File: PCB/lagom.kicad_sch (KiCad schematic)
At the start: 165 parts, among them J1 Conn_01x04, J2 Conn_01x03, SW1 KEYSW, SW10 KEYSW, SW11 KEYSW, SW12 KEYSW, SW13 KEYSW, SW14 KEYSW, SW15 KEYSW, SW16 KEYSW, SW17 KEYSW, SW18 KEYSW, SW19 KEYSW, SW2 KEYSW, SW20 KEYSW, SW21 KEYSW, SW22 KEYSW, SW23 KEYSW, SW24 KEYSW, SW25 KEYSW, SW26 KEYSW, SW27 KEYSW, SW28 KEYSW, SW29 KEYSW, SW3 KEYSW, SW30 KEYSW, SW31 KEYSW, SW32 KEYSW, SW33 KEYSW, SW34 KEYSW, SW35 KEYSW, SW36 KEYSW, SW37 KEYSW, SW38 KEYSW, SW39 KEYSW, SW4 KEYSW, SW40 KEYSW, SW41 KEYSW, SW42 KEYSW, SW43 KEYSW, SW44 KEYSW, SW45 KEYSW, SW46 KEYSW, SW47 KEYSW, SW48 KEYSW, SW49 KEYSW, SW5 KEYSW, SW50 KEYSW, SW51 KEYSW, SW52 KEYSW, SW53 KEYSW, SW54 KEYSW, SW55 KEYSW, SW56 KEYSW, SW57 KEYSW, SW58 KEYSW, SW59 KEYSW, SW6 KEYSW, SW60 KEYSW, SW61 KEYSW, SW62 KEYSW, SW63 KEYSW, SW64 KEYSW, SW65 KEYSW, SW66 KEYSW, SW67 KEYSW, SW68 KEYSW, SW69 KEYSW, SW7 KEYSW, SW70 KEYSW, SW71 KEYSW, SW72 KEYSW, SW73 KEYSW, SW74 KEYSW, SW75 KEYSW, SW76 KEYSW, SW77 KEYSW, SW78 KEYSW, SW79 KEYSW, SW8 KEYSW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

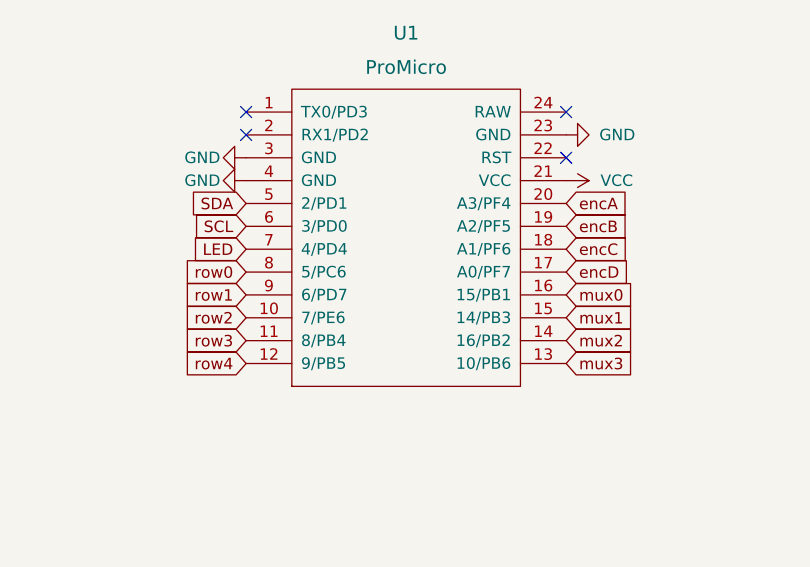
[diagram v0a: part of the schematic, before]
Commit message: PCB mostly done
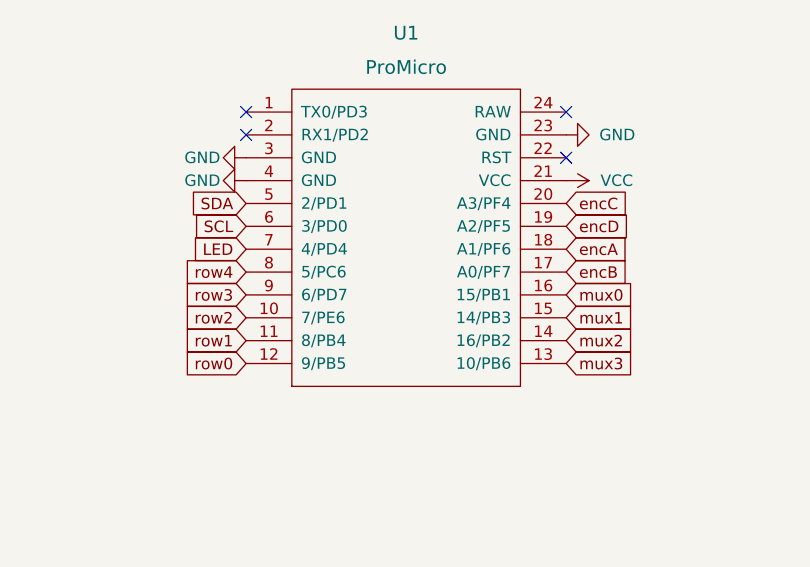
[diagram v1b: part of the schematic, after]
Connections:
- net encA: now also U1.18 (A1/PF6); no longer U1.20 (A3/PF4)
- net encB: now also U1.17 (A0/PF7); no longer U1.19 (A2/PF5)
- net encC: now also U1.20 (A3/PF4); no longer U1.18 (A1/PF6)
- net encD: now also U1.19 (A2/PF5); no longer U1.17 (A0/PF7)
- net row0: now also U1.12 (9/PB5); no longer U1.8 (5/PC6)
- net row1: now also U1.11 (8/PB4); no longer U1.9 (6/PD7)
- net row3: now also U1.9 (6/PD7); no longer U1.11 (8/PB4)
- net row4: now also U1.8 (5/PC6); no longer U1.12 (9/PB5)

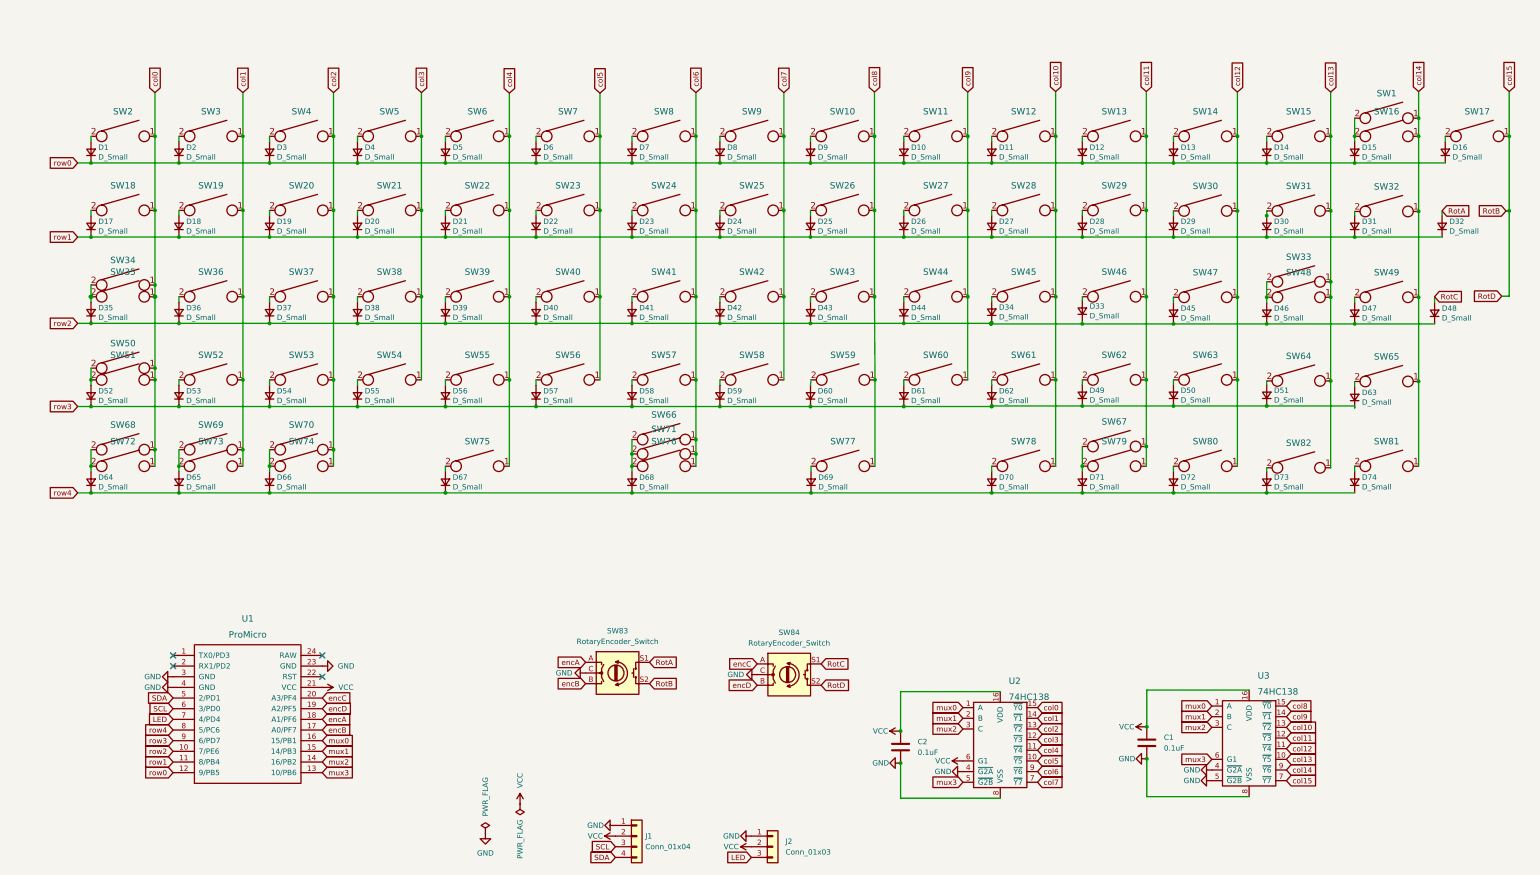
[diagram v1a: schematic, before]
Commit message: Graphics and plate
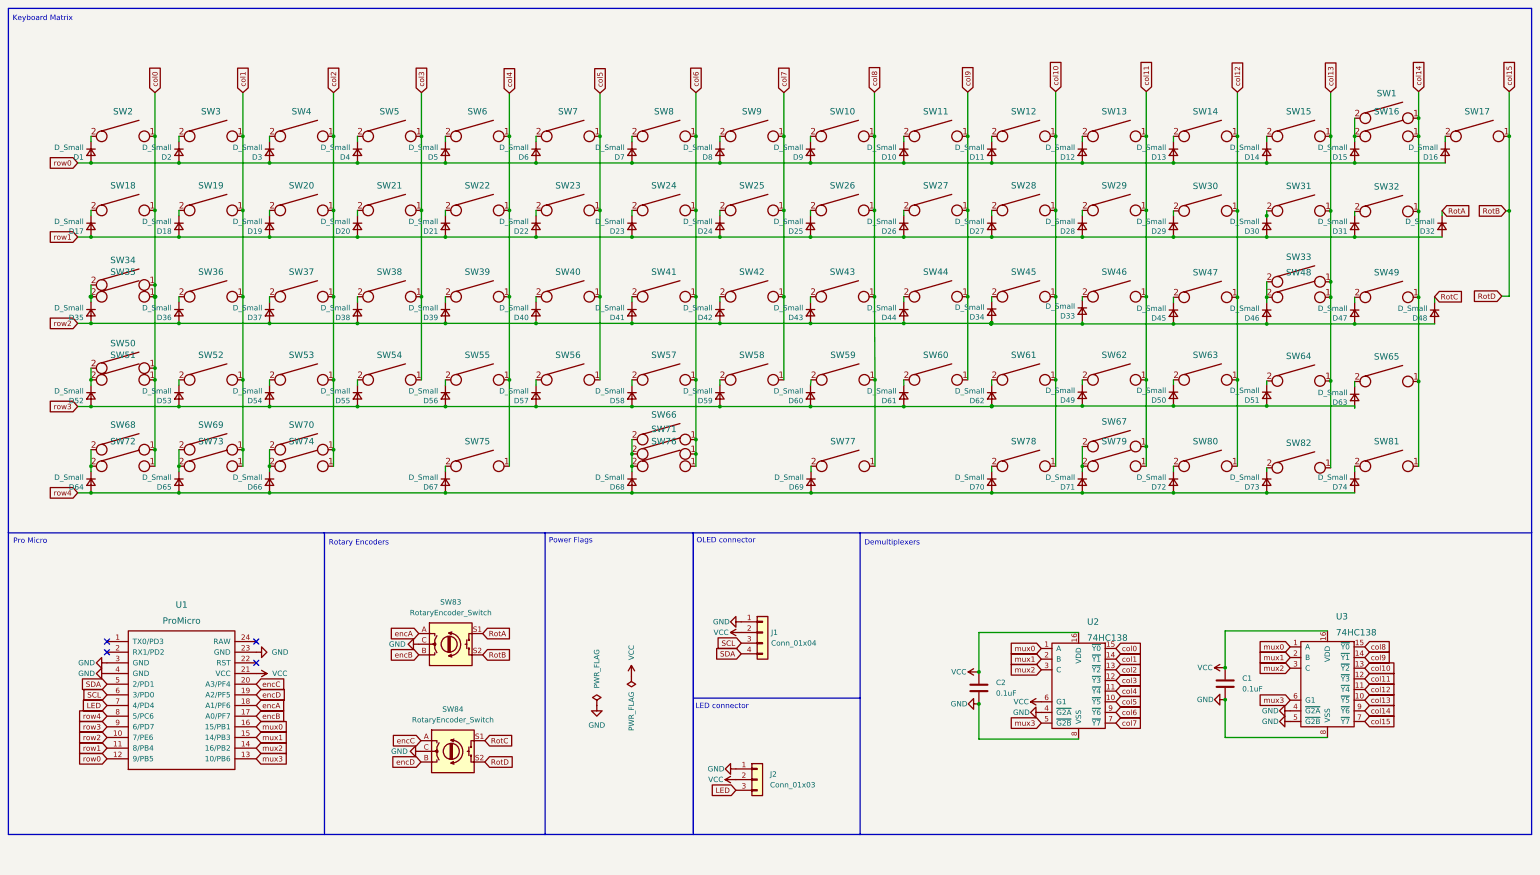
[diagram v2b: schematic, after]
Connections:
- net RotA: now also D32.1 (K); no longer D32.2 (A)
- net RotC: now also D48.1 (K); no longer D48.2 (A)
- net row0: now also D1.2 (A), D10.2 (A), D11.2 (A), D12.2 (A), D13.2 (A), D14.2 (A), D15.2 (A), D16.2 (A), D2.2 (A), D3.2 (A), D4.2 (A), D5.2 (A), D6.2 (A), D7.2 (A), D8.2 (A), D9.2 (A); no longer D1.1 (K), D10.1 (K), D11.1 (K), D12.1 (K), D13.1 (K), D14.1 (K), D15.1 (K), D16.1 (K), D2.1 (K), D3.1 (K), D4.1 (K), D5.1 (K), D6.1 (K), D7.1 (K), D8.1 (K), D9.1 (K)
- net row1: now also D17.2 (A), D18.2 (A), D19.2 (A), D20.2 (A), D21.2 (A), D22.2 (A), D23.2 (A), D24.2 (A), D25.2 (A), D26.2 (A), D27.2 (A), D28.2 (A), D29.2 (A), D30.2 (A), D31.2 (A), D32.2 (A); no longer D17.1 (K), D18.1 (K), D19.1 (K), D20.1 (K), D21.1 (K), D22.1 (K), D23.1 (K), D24.1 (K), D25.1 (K), D26.1 (K), D27.1 (K), D28.1 (K), D29.1 (K), D30.1 (K), D31.1 (K), D32.1 (K)
- net row2: now also D33.2 (A), D34.2 (A), D35.2 (A), D36.2 (A), D37.2 (A), D38.2 (A), D39.2 (A), D40.2 (A), D41.2 (A), D42.2 (A), D43.2 (A), D44.2 (A), D45.2 (A), D46.2 (A), D47.2 (A), D48.2 (A); no longer D33.1 (K), D34.1 (K), D35.1 (K), D36.1 (K), D37.1 (K), D38.1 (K), D39.1 (K), D40.1 (K), D41.1 (K), D42.1 (K), D43.1 (K), D44.1 (K), D45.1 (K), D46.1 (K), D47.1 (K), D48.1 (K)
- net row3: now also D49.2 (A), D50.2 (A), D51.2 (A), D52.2 (A), D53.2 (A), D54.2 (A), D55.2 (A), D56.2 (A), D57.2 (A), D58.2 (A), D59.2 (A), D60.2 (A), D61.2 (A), D62.2 (A), D63.2 (A); no longer D49.1 (K), D50.1 (K), D51.1 (K), D52.1 (K), D53.1 (K), D54.1 (K), D55.1 (K), D56.1 (K), D57.1 (K), D58.1 (K), D59.1 (K), D60.1 (K), D61.1 (K), D62.1 (K), D63.1 (K)
- net row4: now also D64.2 (A), D65.2 (A), D66.2 (A), D67.2 (A), D68.2 (A), D69.2 (A), D70.2 (A), D71.2 (A), D72.2 (A), D73.2 (A), D74.2 (A); no longer D64.1 (K), D65.1 (K), D66.1 (K), D67.1 (K), D68.1 (K), D69.1 (K), D70.1 (K), D71.1 (K), D72.1 (K), D73.1 (K), D74.1 (K)
- net at SW43.2: now also D43.1 (K); no longer D43.2 (A)
- net at SW45.2: now also D34.1 (K); no longer D34.2 (A)
- net at SW5.2: now also D4.1 (K); no longer D4.2 (A)
- net at SW63.2: now also D50.1 (K); no longer D50.2 (A)
- net at SW53.2: now also D54.1 (K); no longer D54.2 (A)
- net at SW2.2: now also D1.1 (K); no longer D1.2 (A)
- net at SW12.2: now also D11.1 (K); no longer D11.2 (A)
- net at SW24.2: now also D23.1 (K); no longer D23.2 (A)
- net at SW18.2: now also D17.1 (K); no longer D17.2 (A)
- net at SW38.2: now also D38.1 (K); no longer D38.2 (A)
- net at SW36.2: now also D36.1 (K); no longer D36.2 (A)
- net at SW44.2: now also D44.1 (K); no longer D44.2 (A)
- net at SW14.2: now also D13.1 (K); no longer D13.2 (A)
- net at SW50.2, SW51.2: now also D52.1 (K); no longer D52.2 (A)
- net at SW28.2: now also D27.1 (K); no longer D27.2 (A)
- net at SW59.2: now also D60.1 (K); no longer D60.2 (A)
- net at SW34.2, SW35.2: now also D35.1 (K); no longer D35.2 (A)
- net at SW26.2: now also D25.1 (K); no longer D25.2 (A)
- net at SW56.2: now also D57.1 (K); no longer D57.2 (A)
- net at SW3.2: now also D2.1 (K); no longer D2.2 (A)
- net at SW13.2: now also D12.1 (K); no longer D12.2 (A)
- net at SW60.2: now also D61.1 (K); no longer D61.2 (A)
- net at SW49.2: now also D47.1 (K); no longer D47.2 (A)
- net at SW31.2: now also D30.1 (K); no longer D30.2 (A)
- net at SW20.2: now also D19.1 (K); no longer D19.2 (A)
- net at SW55.2: now also D56.1 (K); no longer D56.2 (A)
- net at SW10.2: now also D9.1 (K); no longer D9.2 (A)
- net at SW61.2: now also D62.1 (K); no longer D62.2 (A)
- net at SW17.2: now also D16.1 (K); no longer D16.2 (A)
- net at SW42.2: now also D42.1 (K); no longer D42.2 (A)
- net at SW66.2, SW71.2, SW76.2: now also D68.1 (K); no longer D68.2 (A)
- net at SW57.2: now also D58.1 (K); no longer D58.2 (A)
- net at SW27.2: now also D26.1 (K); no longer D26.2 (A)
- net at SW11.2: now also D10.1 (K); no longer D10.2 (A)
- net at SW65.2: now also D63.1 (K); no longer D63.2 (A)
- net at SW8.2: now also D7.1 (K); no longer D7.2 (A)
- net at SW81.2: now also D74.1 (K); no longer D74.2 (A)
- net at SW58.2: now also D59.1 (K); no longer D59.2 (A)
- net at SW69.2, SW73.2: now also D65.1 (K); no longer D65.2 (A)
- net at SW67.2, SW79.2: now also D71.1 (K); no longer D71.2 (A)
- net at SW23.2: now also D22.1 (K); no longer D22.2 (A)
- net at SW39.2: now also D39.1 (K); no longer D39.2 (A)
- net at SW22.2: now also D21.1 (K); no longer D21.2 (A)
- net at SW70.2, SW74.2: now also D66.1 (K); no longer D66.2 (A)
- net at SW75.2: now also D67.1 (K); no longer D67.2 (A)
- net at SW68.2, SW72.2: now also D64.1 (K); no longer D64.2 (A)
- net at SW77.2: now also D69.1 (K); no longer D69.2 (A)
- net at SW32.2: now also D31.1 (K); no longer D31.2 (A)
- net at SW54.2: now also D55.1 (K); no longer D55.2 (A)
- net at SW64.2: now also D51.1 (K); no longer D51.2 (A)
- net at SW19.2: now also D18.1 (K); no longer D18.2 (A)
- net at SW9.2: now also D8.1 (K); no longer D8.2 (A)
- net at SW30.2: now also D29.1 (K); no longer D29.2 (A)
- net at SW47.2: now also D45.1 (K); no longer D45.2 (A)
- net at SW41.2: now also D41.1 (K); no longer D41.2 (A)
- net at SW37.2: now also D37.1 (K); no longer D37.2 (A)
- net at SW6.2: now also D5.1 (K); no longer D5.2 (A)
- net at SW7.2: now also D6.1 (K); no longer D6.2 (A)
- net at SW40.2: now also D40.1 (K); no longer D40.2 (A)
- net at SW1.2, SW16.2: now also D15.1 (K); no longer D15.2 (A)
- net at SW80.2: now also D72.1 (K); no longer D72.2 (A)
- net at SW4.2: now also D3.1 (K); no longer D3.2 (A)
- net at SW15.2: now also D14.1 (K); no longer D14.2 (A)
- net at SW62.2: now also D49.1 (K); no longer D49.2 (A)
- net at SW33.2, SW48.2: now also D46.1 (K); no longer D46.2 (A)
- net at SW82.2: now also D73.1 (K); no longer D73.2 (A)
- net at SW21.2: now also D20.1 (K); no longer D20.2 (A)
- net at SW29.2: now also D28.1 (K); no longer D28.2 (A)
- net at SW52.2: now also D53.1 (K); no longer D53.2 (A)
- net at SW25.2: now also D24.1 (K); no longer D24.2 (A)
- net at SW78.2: now also D70.1 (K); no longer D70.2 (A)
- net at SW46.2: now also D33.1 (K); no longer D33.2 (A)
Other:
- note added: "Demultiplexers"
- note added: "Keyboard Matrix"
- note added: "LED connector"
- note added: "OLED connector"
- note added: "Power Flags"
- note added: "Pro Micro"
- note added: "Rotary Encoders"
- moved on the sheet: C1, C2, D1, D10, D11, D12, D13, D14, D15, D16, D17, D18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
